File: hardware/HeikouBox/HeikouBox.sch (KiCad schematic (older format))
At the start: 4 parts

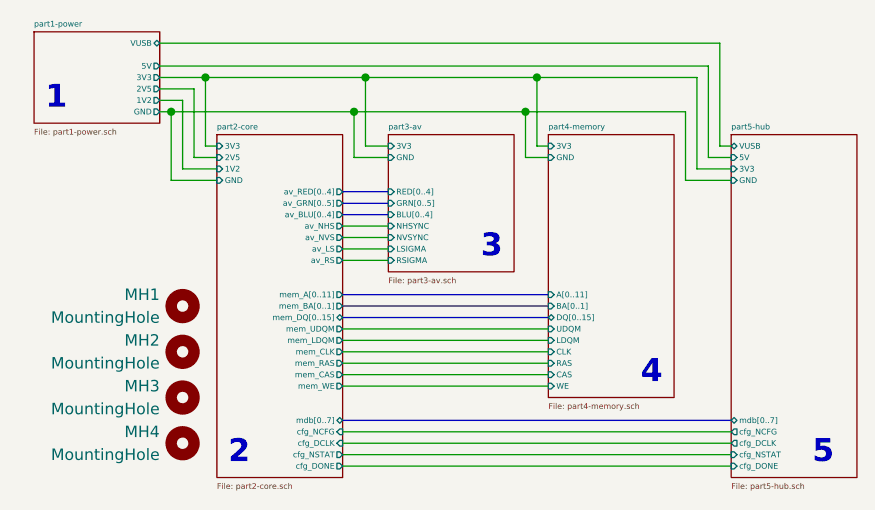
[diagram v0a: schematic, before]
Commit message: More tidy up, move vias
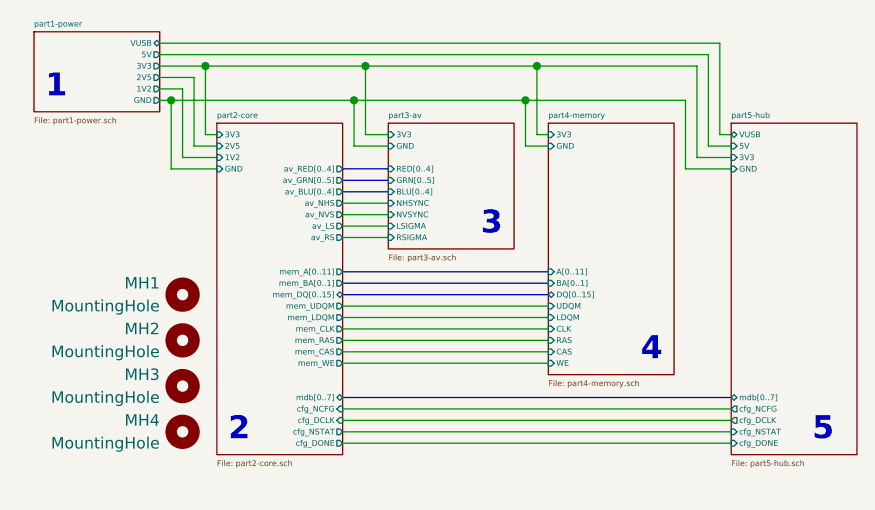
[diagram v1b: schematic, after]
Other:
- moved on the sheet: MH1, MH2, MH3, MH4
